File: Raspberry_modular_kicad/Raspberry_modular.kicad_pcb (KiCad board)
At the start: 2 copper layers, 65 x 56 mm, 93 parts, among them J1 Raspberry_Pi_2_3, U1 MCP3008, U3 MCP3008

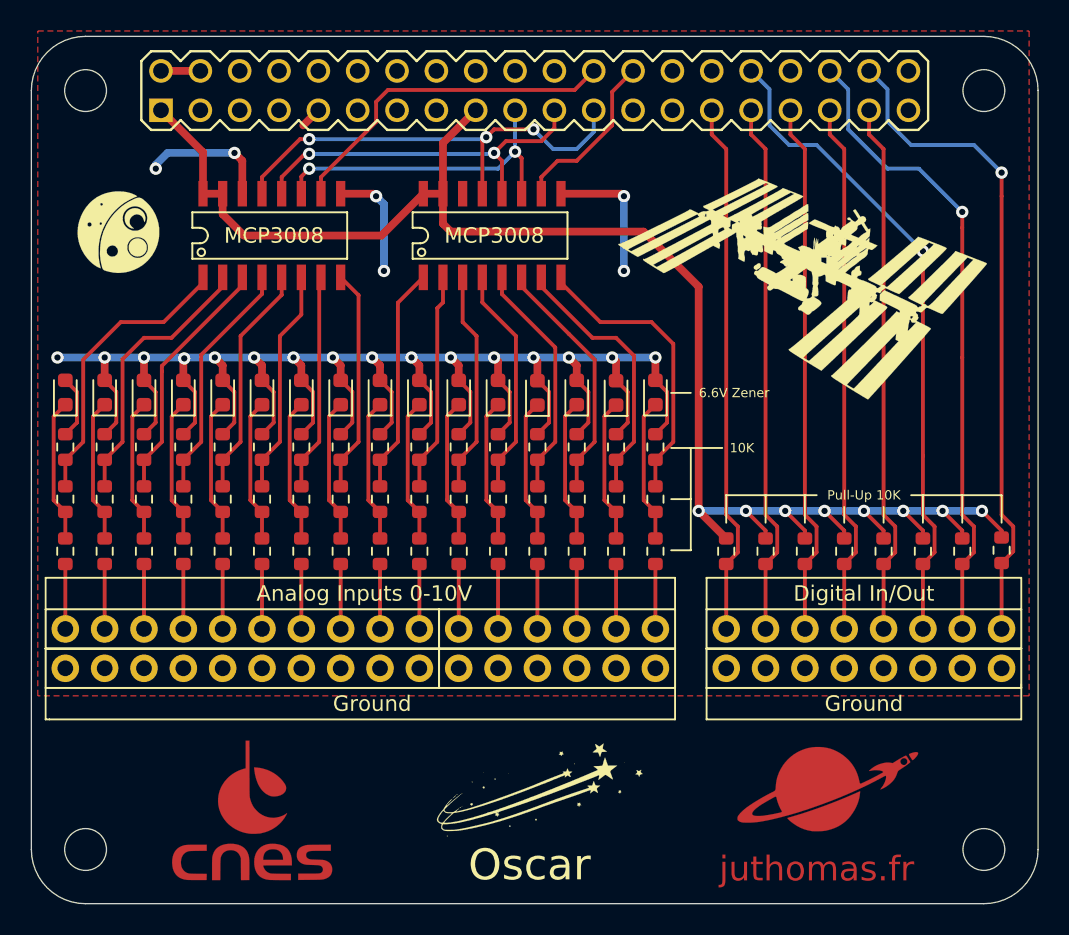
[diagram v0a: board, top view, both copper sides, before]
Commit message: [UDPT] Inputs on schematics
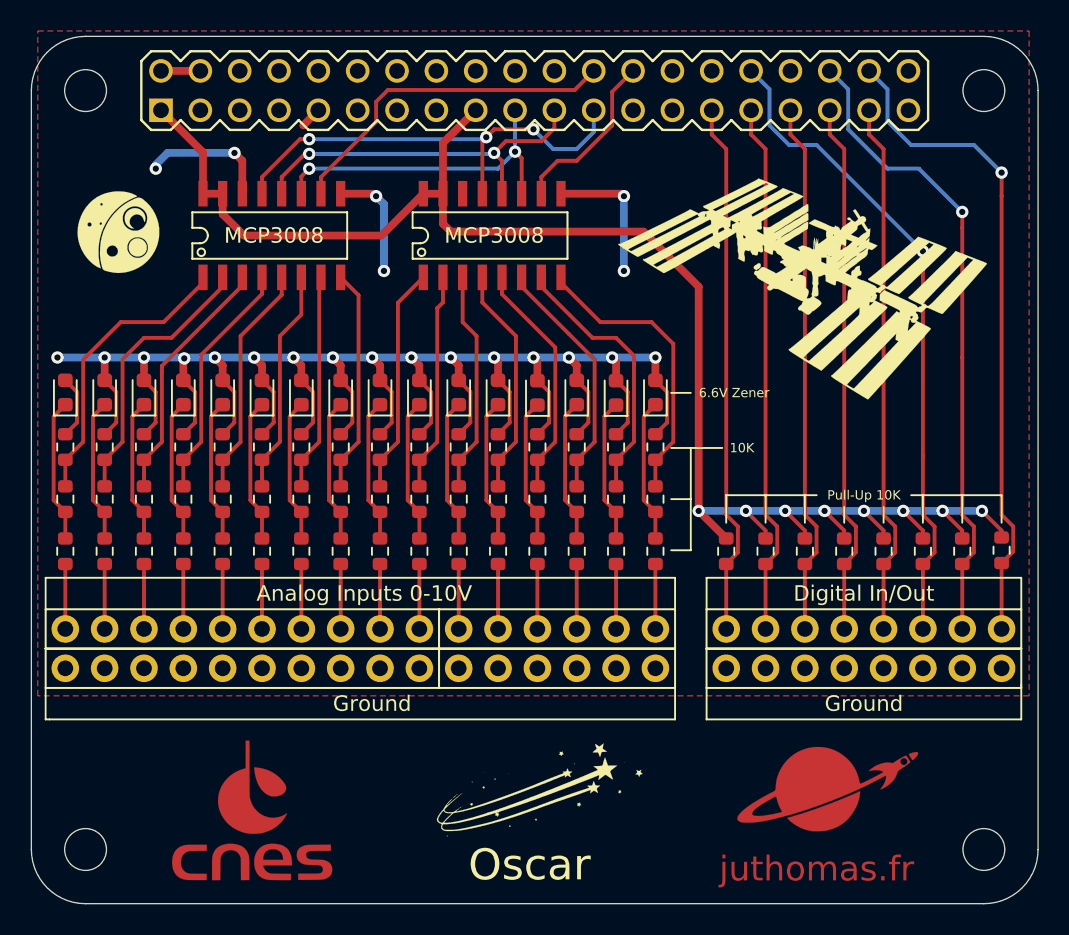
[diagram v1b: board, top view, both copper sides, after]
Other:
- net class Default removed
